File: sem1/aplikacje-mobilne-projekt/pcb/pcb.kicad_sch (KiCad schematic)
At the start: 21 parts, among them J1 Conn_01x20_Female, J2 Conn_01x20_Female, J3 Conn_01x01_Female, J4 Conn_01x01_Female, Q1 IRL6283M, Q10 IRL6283M, Q11 IRL6283M, Q12 IRL6283M, Q13 IRL6283M, Q2 IRL6283M, Q3 IRL6283M, Q4 IRL6283M, Q5 IRL6283M, Q6 IRL6283M, Q7 IRL6283M, Q8 IRL6283M, Q9 IRL6283M

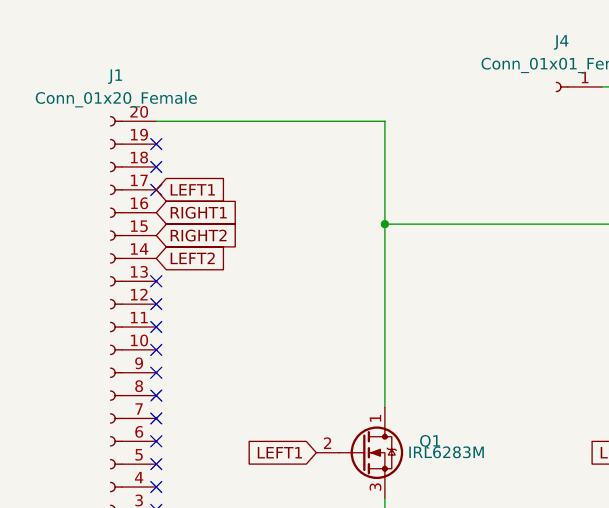
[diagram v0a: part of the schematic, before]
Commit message: kicad schematic
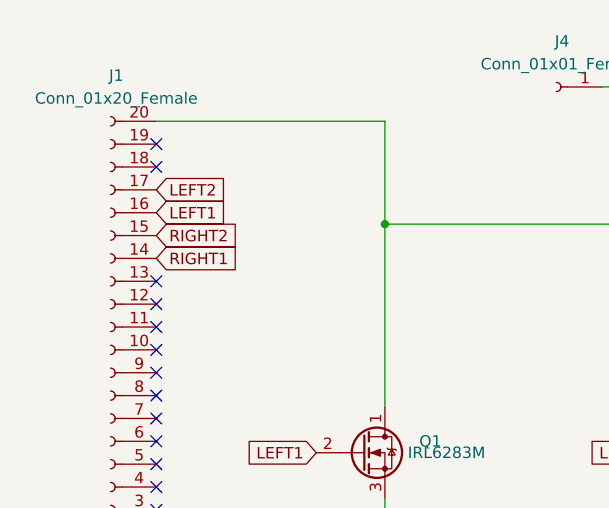
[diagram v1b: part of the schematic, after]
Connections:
- net LEFT1: now also J1.16 (Pin_16); no longer J1.17 (Pin_17)
- net LEFT2: now also J1.17 (Pin_17); no longer J1.14 (Pin_14)
- net RIGHT1: now also J1.14 (Pin_14); no longer J1.16 (Pin_16)
- no-connect marks 35 -> 34
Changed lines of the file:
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@@
   (no_connect (at 40.64 81.28))
   (no_connect (at 40.64 140.97))
-  (no_connect (at 40.64 40.64))
   (no_connect (at 40.64 68.58))
   (no_connect (at 40.64 125.73))
@@
     (stroke (width 0) (type default) (color 0 0 0 0))
   )
-  (global_label "RIGHT1" (shape input) (at 40.64 43.18 0) (fields_autoplaced)
-    (effects (font (size 1.27 1.27)) (justify left))
-    (property "Intersheet References" "${INTERSHEET_REFS}" (id 0) (at 49.7055 43.1006 0)
-      (effects (font (size 1.27 1.27)) (justify left) hide)
-    )
-  )
   (global_label "RIGHT1" (shape input) (at 191.77 107.95 180) (fields_autoplaced)
     (effects (font (size 1.27 1.27)) (justify right))
@@
     )
   )
+  (global_label "LEFT1" (shape input) (at 40.64 43.18 0) (fields_autoplaced)
+    (effects (font (size 1.27 1.27)) (justify left))
+    (property "Intersheet References" "${INTERSHEET_REFS}" (id 0) (at 48.496 43.2594 0)
+      (effects (font (size 1.27 1.27)) (justify left) hide)
+    )
+  )
   (global_label "Gnd" (shape input) (at 247.65 113.03 270) (fields_autoplaced)
     (effects (font (size 1.27 1.27)) (justify right))
@@
     )
   )
+  (global_label "LEFT2" (shape input) (at 40.64 40.64 0) (fields_autoplaced)
+    (effects (font (size 1.27 1.27)) (justify left))
+    (property "Intersheet References" "${INTERSHEET_REFS}" (id 0) (at 48.496 40.7194 0)
+      (effects (font (size 1.27 1.27)) (justify left) hide)
+    )
+  )
   (global_label "RIGHT2" (shape input) (at 40.64 45.72 0) (fields_autoplaced)
     (effects (font (size 1.27 1.27)) (justify left))
@@
     )
   )
-  (global_label "LEFT1" (shape input) (at 40.64 40.64 0) (fields_autoplaced)
-    (effects (font (size 1.27 1.27)) (justify left))
-    (property "Intersheet References" "${INTERSHEET_REFS}" (id 0) (at 48.496 40.7194 0)
+  (global_label "RIGHT1" (shape input) (at 40.64 48.26 0) (fields_autoplaced)
+    (effects (font (size 1.27 1.27)) (justify left))
+    (property "Intersheet References" "${INTERSHEET_REFS}" (id 0) (at 49.7055 48.1806 0)
       (effects (font (size 1.27 1.27)) (justify left) hide)
     )
@@
     )
   )
-  (global_label "LEFT2" (shape input) (at 40.64 48.26 0) (fields_autoplaced)
-    (effects (font (size 1.27 1.27)) (justify left))
-    (property "Intersheet References" "${INTERSHEET_REFS}" (id 0) (at 48.496 48.3394 0)
-      (effects (font (size 1.27 1.27)) (justify left) hide)
-    )
-  )
